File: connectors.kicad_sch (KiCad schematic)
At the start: 34 parts, among them J10 Conn_01x02, J11 Conn_01x02, J12 Conn_01x02, J13 USB_C_Receptacle_PowerOnly_6P, J14 USB_C_Receptacle_USB2.0_16P, J15 USB_C_Receptacle_USB2.0_16P, J3 VIN, J4 Conn_01x08, J5 Conn_01x08, J6 Conn_01x08, J7 Conn_01x02, J8 Conn_01x02, J9 Conn_01x02

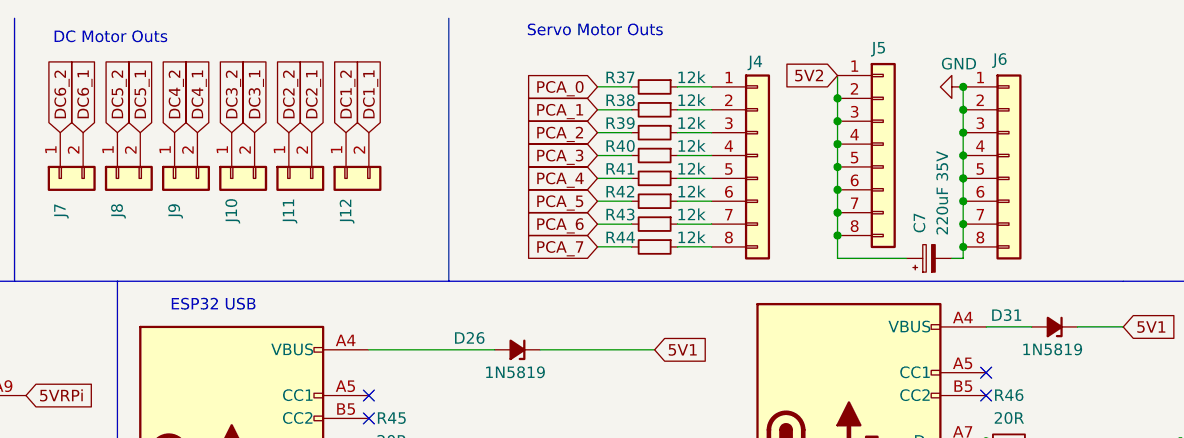
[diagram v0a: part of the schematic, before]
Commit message: Revert "placing completed."
This reverts commit 8fc8ab54a7d5bb0e004d046318c33d8a5f2fb8c8.
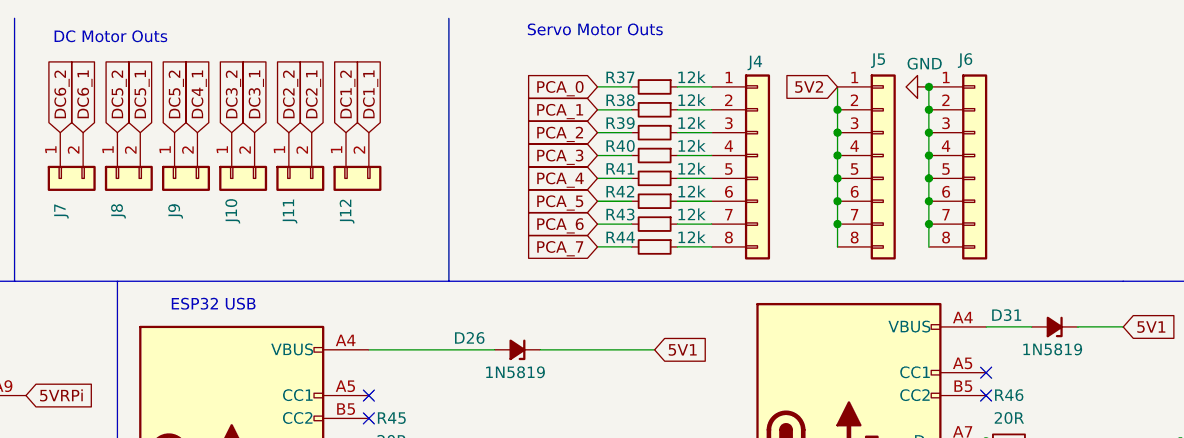
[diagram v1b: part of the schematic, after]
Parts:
- removed C7: 220uF 35V, Capacitor_SMD:CP_Elec_8x10.5, symbol Device:C_Polarized_Small
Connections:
- net DC4_2 is gone; now on net DC5_2: J9.1 (Pin_1)
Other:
- moved on the sheet: J5, J6
